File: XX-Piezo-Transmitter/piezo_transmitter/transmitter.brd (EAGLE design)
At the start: 26.9 x 24.6 mm, 7 parts, among them U1 BD6221FSOP, U2 ATTINY24A-SSUR

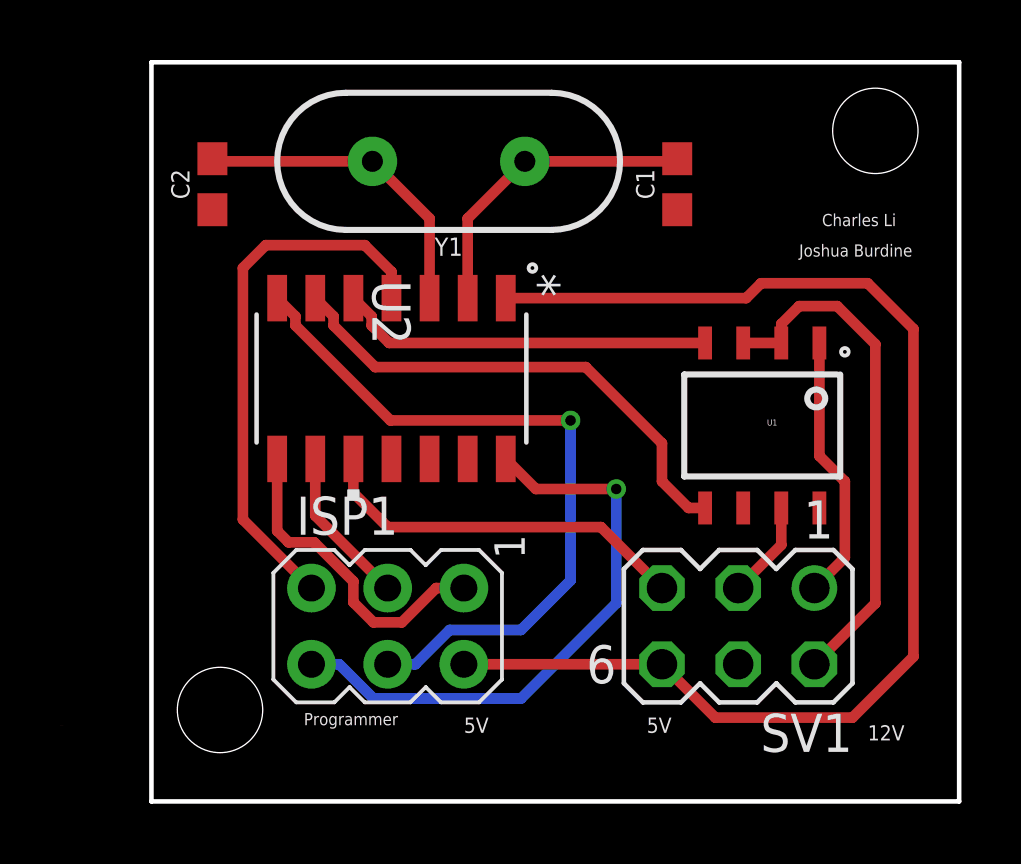
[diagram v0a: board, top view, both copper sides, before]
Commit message: Fixed trace names
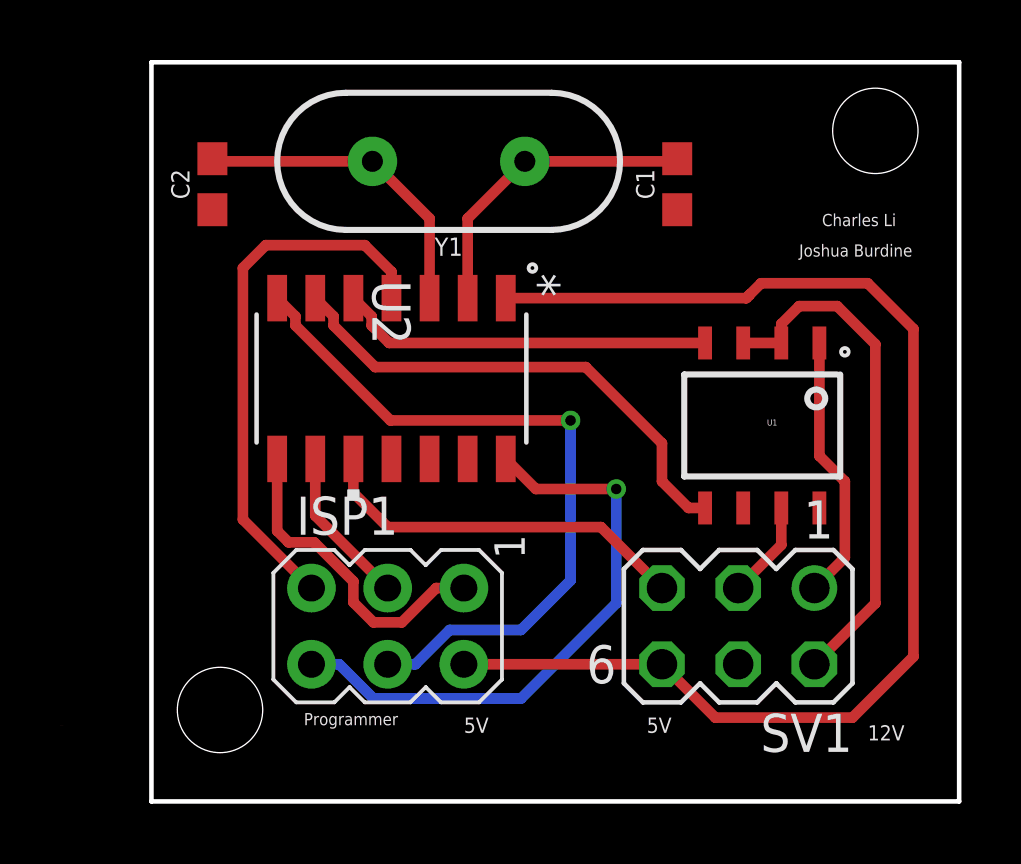
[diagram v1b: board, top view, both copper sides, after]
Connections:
- net N$10 renamed RIN
- net N$11 renamed SCK
- net N$12 renamed MISO
- net N$2 renamed XTAL1
- net N$3 renamed XTAL2
- net N$4 renamed MOSI
- net N$5 renamed IO
- net N$6 renamed RESET
- net N$7 renamed PIEZO+
- net N$8 renamed PIEZO-
- net N$9 renamed FIN
- net VCC renamed 12V
- net VCC_2 renamed 5V
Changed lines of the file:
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@@
 </elements>
 <signals>
-<signal name="VCC">
-<contactref element="U1" pad="2"/>
-<contactref element="U1" pad="3"/>
-<wire x1="22.773" y1="12.742" x2="24.043" y2="12.742" width="0.3556" layer="1"/>
-<contactref element="SV1" pad="2"/>
-<wire x1="24.043" y1="12.742" x2="24.043" y2="13.375" width="0.3556" layer="1"/>
-<wire x1="24.043" y1="13.375" x2="24.638" y2="13.97" width="0.3556" layer="1"/>
-<wire x1="24.638" y1="13.97" x2="25.908" y2="13.97" width="0.3556" layer="1"/>
-<wire x1="25.908" y1="13.97" x2="27.178" y2="12.7" width="0.3556" layer="1"/>
-<wire x1="27.178" y1="12.7" x2="27.178" y2="4.064" width="0.3556" layer="1"/>
-<wire x1="27.178" y1="4.064" x2="25.146" y2="2.032" width="0.3556" layer="1"/>
-</signal>
 <signal name="GND">
 <contactref element="U2" pad="14"/>
 <contactref element="ISP1" pad="6"/>
 <contactref element="U1" pad="8"/>
-<contactref element="C1" pad="1"/>
-<contactref element="C2" pad="1"/>
 <contactref element="SV1" pad="4"/>
 <wire x1="14.859" y1="8.8773" x2="15.8623" y2="7.874" width="0.3556" layer="1"/>
@@
 <vertex x="3.048" y="-2.54"/>
 </polygon>
-</signal>
-<signal name="VCC_2">
-<contactref element="U2" pad="1"/>
-<contactref element="ISP1" pad="2"/>
-<contactref element="SV1" pad="6"/>
-<wire x1="20.066" y1="2.032" x2="13.462" y2="2.032" width="0.3556" layer="1"/>
-<wire x1="14.859" y1="14.2367" x2="22.8727" y2="14.2367" width="0.3556" layer="1"/>
-<wire x1="22.8727" y1="14.2367" x2="23.368" y2="14.732" width="0.3556" layer="1"/>
-<wire x1="23.368" y1="14.732" x2="26.924" y2="14.732" width="0.3556" layer="1"/>
-<wire x1="26.924" y1="14.732" x2="28.448" y2="13.208" width="0.3556" layer="1"/>
-<wire x1="28.448" y1="13.208" x2="28.448" y2="2.286" width="0.3556" layer="1"/>
-<wire x1="28.448" y1="2.286" x2="26.416" y2="0.254" width="0.3556" layer="1"/>
-<wire x1="26.416" y1="0.254" x2="21.844" y2="0.254" width="0.3556" layer="1"/>
-<wire x1="21.844" y1="0.254" x2="20.066" y2="2.032" width="0.3556" layer="1"/>
+<contactref element="C1" pad="1"/>
+<contactref element="C2" pad="1"/>
 </signal>
 <signal name="N$1">
 </signal>
-<signal name="N$2">
+<signal name="XTAL1">
 <contactref element="U2" pad="2"/>
 <contactref element="Y1" pad="1"/>
 <contactref element="C1" pad="2"/>
 <wire x1="13.589" y1="14.605" x2="13.589" y2="14.2367" width="0.3556" layer="1"/>
-<wire x1="13.589" y1="14.2367" x2="13.589" y2="16.891" width="0.3556" layer="1"/>
 <wire x1="13.589" y1="16.891" x2="15.494" y2="18.796" width="0.3556" layer="1"/>
 <wire x1="15.494" y1="18.796" x2="20.486" y2="18.796" width="0.3556" layer="1"/>
 <wire x1="20.486" y1="18.796" x2="20.574" y2="18.884" width="0.3556" layer="1"/>
+<wire x1="13.589" y1="14.2367" x2="13.589" y2="16.891" width="0.3556" layer="1"/>
 </signal>
-<signal name="N$3">
+<signal name="XTAL2">
 <contactref element="U2" pad="3"/>
 <contactref element="Y1" pad="2"/>
@@
 <wire x1="5.168" y1="18.796" x2="5.08" y2="18.884" width="0.3556" layer="1"/>
 </signal>
-<signal name="N$4">
+<signal name="MOSI">
 <contactref element="U2" pad="7"/>
 <contactref element="ISP1" pad="4"/>
@@
 <wire x1="12.98855" y1="3.175" x2="11.84555" y2="2.032" width="0.3556" layer="16"/>
 </signal>
-<signal name="N$6">
+<signal name="RESET">
 <contactref element="U2" pad="4"/>
 <contactref element="ISP1" pad="5"/>
@@
 <wire x1="6.096" y1="6.858" x2="8.382" y2="4.572" width="0.3556" layer="1"/>
 </signal>
-<signal name="N$5">
+<signal name="IO">
 <contactref element="U2" pad="10"/>
 <contactref element="SV1" pad="5"/>
@@
 <wire x1="18.034" y1="6.604" x2="20.066" y2="4.572" width="0.3556" layer="1"/>
 </signal>
-<signal name="N$7">
+<signal name="PIEZO+">
 <contactref element="U1" pad="1"/>
 <contactref element="SV1" pad="1"/>
@@
 <wire x1="26.162" y1="5.588" x2="25.146" y2="4.572" width="0.3556" layer="1"/>
 </signal>
-<signal name="N$8">
+<signal name="PIEZO-">
 <contactref element="U1" pad="7"/>
 <contactref element="SV1" pad="3"/>
@@
 <wire x1="24.043" y1="6.009" x2="24.043" y2="7.242" width="0.3556" layer="1"/>
 </signal>
-<signal name="N$9">
+<signal name="FIN">
 <contactref element="U2" pad="5"/>
 <contactref element="U1" pad="4"/>
@@
 <wire x1="10.971825" y1="12.742" x2="21.503" y2="12.742" width="0.3556" layer="1"/>
 </signal>
-<signal name="N$10">
+<signal name="RIN">
 <contactref element="U2" pad="6"/>
 <contactref element="U1" pad="5"/>
@@
 <wire x1="20.952" y1="7.242" x2="21.503" y2="7.242" width="0.3556" layer="1"/>
 </signal>
-<signal name="N$11">
+<signal name="SCK">
 <contactref element="U2" pad="9"/>
 <contactref element="ISP1" pad="3"/>
@@
 <wire x1="8.509" y1="6.985" x2="8.509" y2="8.8773" width="0.3556" layer="1"/>
 </signal>
-<signal name="N$12">
+<signal name="MISO">
 <contactref element="ISP1" pad="1"/>
 <contactref element="U2" pad="8"/>
@@
 <wire x1="7.239" y1="6.477" x2="7.239" y2="8.8773" width="0.3556" layer="1"/>
 </signal>
+<signal name="5V">
+<contactref element="U2" pad="1"/>
+<contactref element="ISP1" pad="2"/>
+<contactref element="SV1" pad="6"/>
+<wire x1="20.066" y1="2.032" x2="13.462" y2="2.032" width="0.3556" layer="1"/>
+<wire x1="22.987" y1="14.351" x2="22.8727" y2="14.2367" width="0.3556" layer="1"/>
+<wire x1="22.987" y1="14.351" x2="23.368" y2="14.732" width="0.3556" layer="1"/>
+<wire x1="23.368" y1="14.732" x2="26.924" y2="14.732" width="0.3556" layer="1"/>
+<wire x1="26.924" y1="14.732" x2="28.448" y2="13.208" width="0.3556" layer="1"/>
+<wire x1="28.448" y1="13.208" x2="28.448" y2="2.286" width="0.3556" layer="1"/>
+<wire x1="28.448" y1="2.286" x2="26.416" y2="0.254" width="0.3556" layer="1"/>
+<wire x1="26.416" y1="0.254" x2="21.844" y2="0.254" width="0.3556" layer="1"/>
+<wire x1="21.844" y1="0.254" x2="20.066" y2="2.032" width="0.3556" layer="1"/>
+<wire x1="14.859" y1="14.2367" x2="22.8727" y2="14.2367" width="0.3556" layer="1"/>
+<wire x1="22.8727" y1="14.2367" x2="22.987" y2="14.351" width="0.3556" layer="1"/>
+</signal>
+<signal name="12V">
+<contactref element="SV1" pad="2"/>
+<contactref element="U1" pad="2"/>
+<contactref element="U1" pad="3"/>
+<wire x1="22.773" y1="12.742" x2="24.043" y2="12.742" width="0.3556" layer="1"/>
+<wire x1="24.043" y1="12.742" x2="24.043" y2="13.375" width="0.3556" layer="1"/>
+<wire x1="24.043" y1="13.375" x2="24.638" y2="13.97" width="0.3556" layer="1"/>
+<wire x1="24.638" y1="13.97" x2="25.908" y2="13.97" width="0.3556" layer="1"/>
+<wire x1="25.908" y1="13.97" x2="27.178" y2="12.7" width="0.3556" layer="1"/>
+<wire x1="27.178" y1="4.064" x2="27.178" y2="12.7" width="0.3556" layer="1"/>
+<wire x1="25.146" y1="2.032" x2="27.178" y2="4.064" width="0.3556" layer="1"/>
+</signal>
 </signals>
